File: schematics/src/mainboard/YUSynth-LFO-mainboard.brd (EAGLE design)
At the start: 160 x 100 mm, 42 parts, among them IC1 TL074P, IC2 TL074P, IC3 NE555N

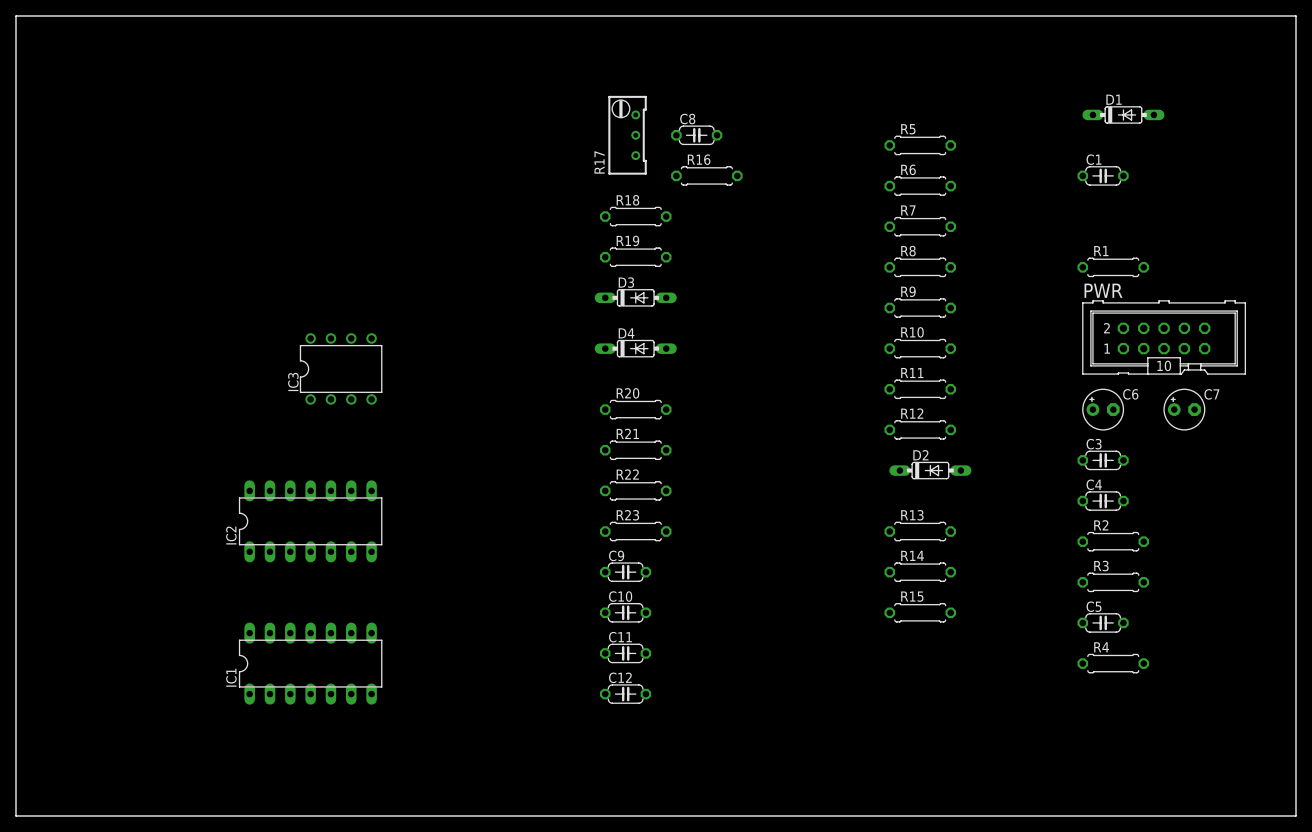
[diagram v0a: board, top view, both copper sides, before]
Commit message: initial designs
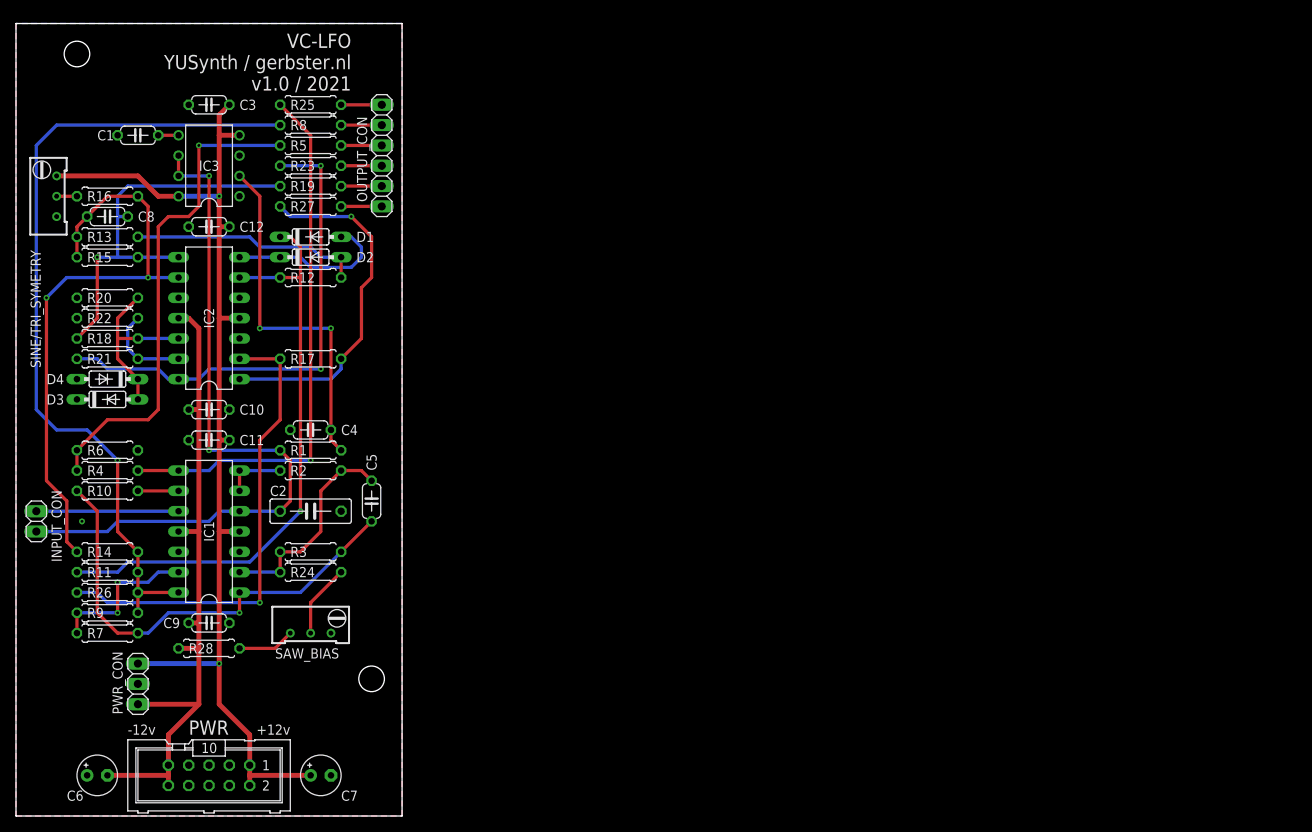
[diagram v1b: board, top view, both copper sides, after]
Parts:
- added C2: 1uF, rcl:C075-032X103
- added INPUT_CON: (no value), pinhead:1X02
- added OUTPUT_CON: (no value), pinhead:1X06
- added PWR_CON: (no value), pinhead:1X03
- added R24, R26: 100k, rcl:0207/7
- added R25: 47k, rcl:0207/7
- added R27: 1k, rcl:0207/7
- added R28: 2.7k, rcl:0207/7
- added SAW_BIAS: 10k, rcl:RTRIM64W
- added SINE/TRI_SYMETRY: 50k, rcl:RTRIM64W
- C1: value (none) -> 10nF
- C10, C11, C12, C3, C9: value (none) -> .1uF
- C4: value (none) -> 47nF
- C5: value (none) -> 120pF
- C8: value (none) -> 1nF
- D1, D2, D3, D4: value 4148 -> 1n4148
- R1, R19, R23, R5, R8: value (none) -> 1k
- R10, R6: value (none) -> 10k
- R11, R12, R14, R2: value (none) -> 100k/1%
- R13: value (none) -> 50k/1%
- R15, R3: value (none) -> 200k/1%
- R16, R18: value (none) -> 150k
- R17: value (none) -> 100k; device rcl:RTRIM64W -> rcl:0207/7
- R20: value (none) -> 22k
- R21: value (none) -> 15k
- R22: value (none) -> 1.5k
- R4: value (none) -> 12k
- R7: value (none) -> 120k
- R9: value (none) -> 100k
- moved C6 133.8 mm to (10.2, 5.08)
- moved PWR 131.3 mm to (24.1, 5.08), turned to 180 degrees
- moved R4 128.0 mm to (11.4, 43.2), turned to 180 degrees
- moved C1 120.8 mm to (15.2, 85.1), turned to 180 degrees
- moved C3 120.3 mm to (24.1, 88.9), turned to 180 degrees
- moved C7 117.2 mm to (38.1, 5.08)
- moved R7 113.6 mm to (11.4, 22.9), turned to 180 degrees
- moved R15 110.9 mm to (11.4, 69.8)
- moved R9 108.5 mm to (11.4, 25.4)
- moved R13 108.1 mm to (11.4, 72.4)
- moved R6 106.8 mm to (11.4, 45.7), turned to 180 degrees
- moved R11 104.1 mm to (11.4, 30.5), turned to 180 degrees
- moved R10 103.1 mm to (11.4, 40.6)
- moved R1 102.9 mm to (36.8, 45.7)
- moved D1 102.7 mm to (36.8, 72.4)
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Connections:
- removed net CV_INPUT: IC1.5, IC3.6, IC3.7, R1.1
- new net CV: C2.1, IC1.5, IC3.6, IC3.7, INPUT_CON.1, R1.1
- new net LED: OUTPUT_CON.6, R25.2
- new net N$21: IC1.14, R11.1, R14.1, R26.1, R8.1, R9.2
- new net N$23: IC2.1, R17.2, R27.1
- new net N$5: IC2.2, R17.1, R26.2
- new net RAMP_OUT: OUTPUT_CON.1, R27.2
- net +12V: now also PWR_CON.1, SINE/TRI_SYMETRY.3; no longer R17.3
- net -12V: now also PWR_CON.3, R28.2
- net GND: now also C2.2, PWR_CON.2, SAW_BIAS.3, SINE/TRI_SYMETRY.1; no longer R17.1
- net LED_OUT: now also R25.1
- net N$10: now also R28.1, SAW_BIAS.1; no longer IC2.1, IC2.2
- net N$16: now also SINE/TRI_SYMETRY.2; no longer R17.2
- net N$4: now also R24.2
- net N$7: now also R24.1, SAW_BIAS.2; no longer IC1.14, R8.1, R9.2
- net N$8: no longer R11.1, R14.1
- net PULSE_OUT: now also OUTPUT_CON.4
- net PULSE_WIDTH: now also INPUT_CON.2
- net SAW_OUT: now also OUTPUT_CON.5
- net SINE_OUT: now also OUTPUT_CON.3
- net TRI_OUT: now also OUTPUT_CON.2
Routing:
- net +12V: track 0.00 -> 136.5 mm, vias 0 -> 2
- net N$21: track 0.00 -> 102.5 mm, vias 0 -> 1
- net CV: track 0.00 -> 89.7 mm, vias 0 -> 2
- net -12V: track 0.00 -> 84.7 mm
- net N$12: track 0.00 -> 74.8 mm, vias 0 -> 1
- net N$13: track 0.00 -> 74.6 mm, vias 0 -> 2
- net LED_OUT: track 0.00 -> 68.1 mm, vias 0 -> 1
- net N$19: track 0.00 -> 62.5 mm, vias 0 -> 2
- net N$6: track 0.00 -> 61.6 mm, vias 0 -> 1
- net N$5: track 0.00 -> 60.0 mm, vias 0 -> 1
- net N$8: track 0.00 -> 58.9 mm, vias 0 -> 1
- net N$17: track 0.00 -> 51.1 mm, vias 0 -> 1
- net N$2: track 0.00 -> 44.8 mm, vias 0 -> 2
- net N$23: track 0.00 -> 44.3 mm, vias 0 -> 1
- net N$15: track 0.00 -> 29.0 mm
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- added copper zone on layer 1, net GND
- added copper zone on layer 16, net GND
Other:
- board size 160 x 100 mm -> 48.3 x 99.1 mm
- board text added: "+12v"
- board text added: "-12v"
- board text added: "VC-LFO YUSynth / gerbster.nl v1.0 / 2021"
